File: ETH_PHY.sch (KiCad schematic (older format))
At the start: 19 parts

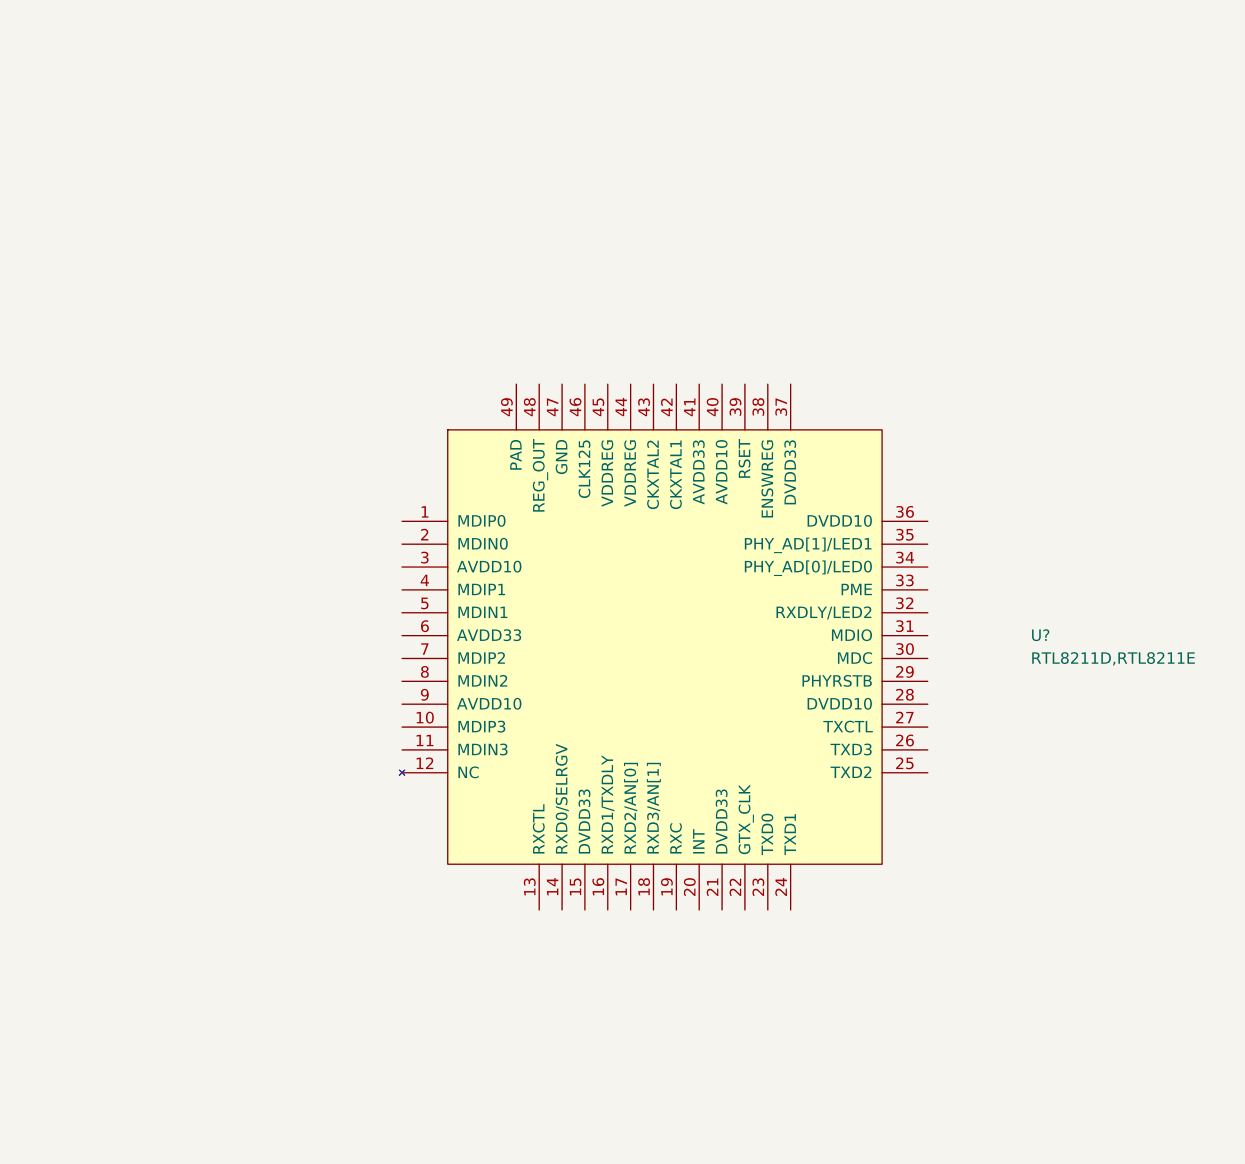
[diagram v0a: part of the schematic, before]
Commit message: update for EPHY,
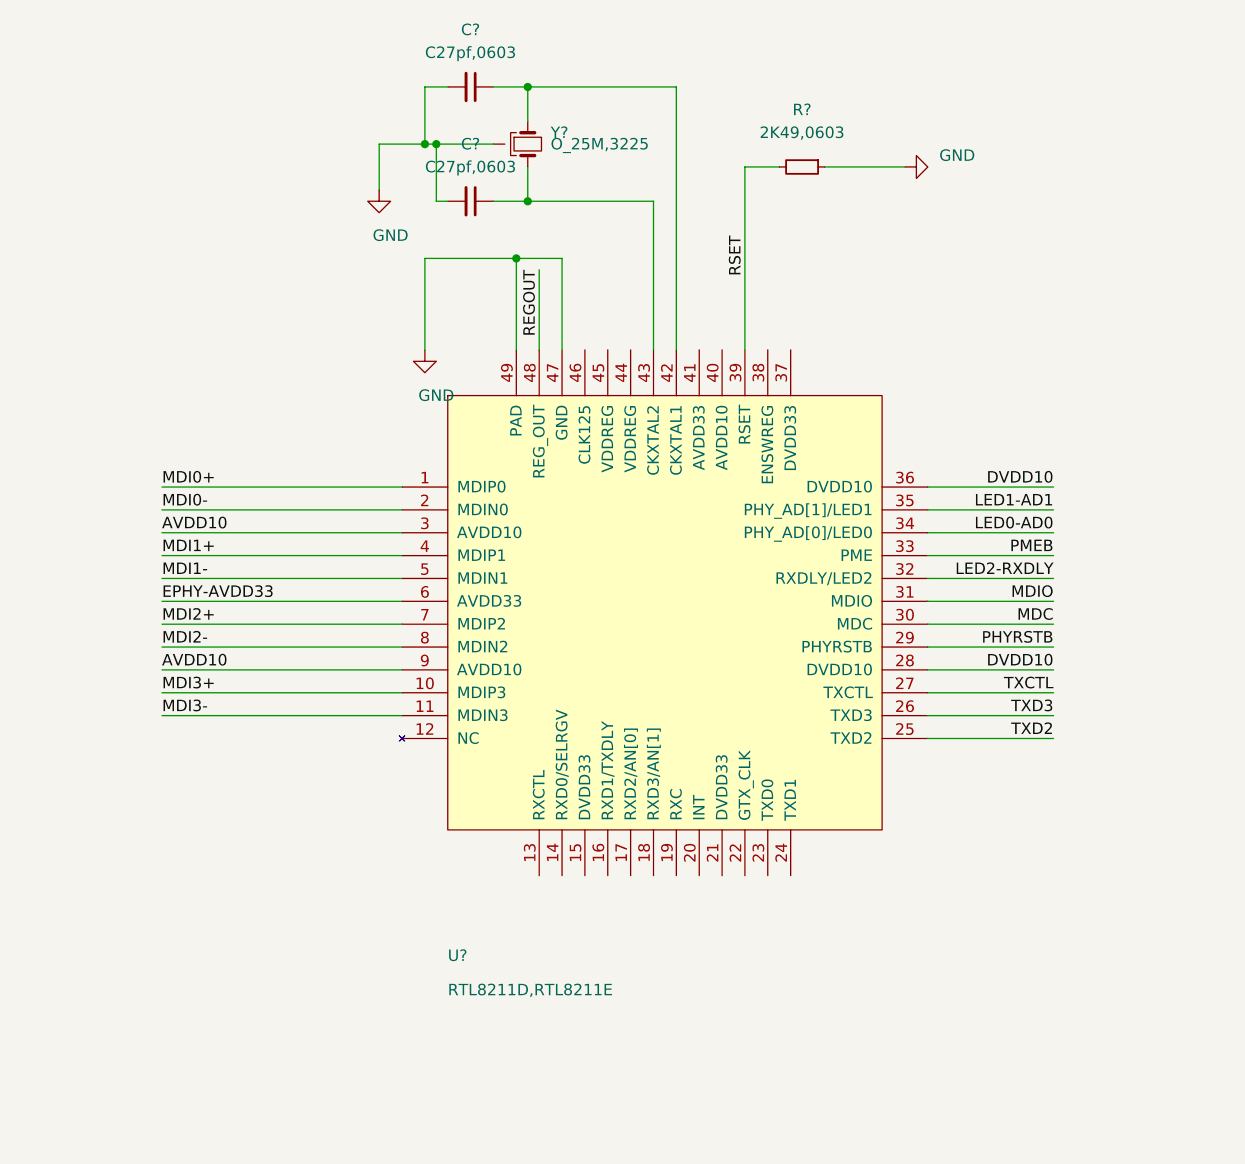
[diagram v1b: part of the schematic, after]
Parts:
- removed U?: RTL8211D,RTL8211E, symbol taobao-components:RTL8211D,RTL8211E
- added C? (x2): C27pf,0603, Capacitor_SMD:C_0603_1608Metric_Pad1.05x0.95mm_HandSolder, symbol taobao-c:C27pf,0603
- added R?: 2K49,0603, symbol Device:R_Small
- added U?: RTL8211D,RTL8211E, symbol taobao-components:RTL8211D,RTL8211E
- added Y?: O_25M,3225, Oscillator:Oscillator_SMD_Abracon_ASE-4Pin_3.2x2.5mm_HandSoldering, symbol taobao-osc:O_25M,3225
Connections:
- net GND: now also C?.2, C?.2, R?.1, U?.47 (GND), U?.49 (PAD), Y?.2
- new net: C?.1, U?.42 (CKXTAL1), Y?.1
- new net: C?.1, U?.43 (CKXTAL2), Y?.3
- new net AVDD10: U?.3 (AVDD10), U?.9 (AVDD10)
- new net DVDD10: U?.28 (DVDD10), U?.36 (DVDD10)
- new net EPHY-AVDD33: U?.6 (AVDD33)
- new net LED0-AD0: U?.34 (PHY_AD[0]/LED0)
- new net LED1-AD1: U?.35 (PHY_AD[1]/LED1)
- new net LED2-RXDLY: U?.32 (RXDLY/LED2)
- new net MDC: U?.30 (MDC)
- new net MDI0+: U?.1 (MDIP0)
- new net MDI0-: U?.2 (MDIN0)
- new net MDI1+: U?.4 (MDIP1)
- new net MDI1-: U?.5 (MDIN1)
- new net MDI2+: U?.7 (MDIP2)
- new net MDI2-: U?.8 (MDIN2)
- new net MDI3+: U?.10 (MDIP3)
- new net MDI3-: U?.11 (MDIN3)
- new net MDIO: U?.31 (MDIO)
- new net PHYRSTB: U?.29 (PHYRSTB)
- new net PMEB: U?.33 (PME)
- new net REGOUT: U?.48 (REG_OUT)
- new net RSET: R?.2, U?.39 (RSET)
- new net TXCTL: U?.27 (TXCTL)
- new net TXD2: U?.25 (TXD2)
- new net TXD3: U?.26 (TXD3)
